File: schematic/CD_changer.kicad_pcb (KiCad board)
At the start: 2 copper layers, 27 parts, among them J1 Mini-ISO_Conn, J2 Prog, SW1 Enable, SW2 SW_Reset, U1 ESP32-WROOM-32, U3 PCM5102A

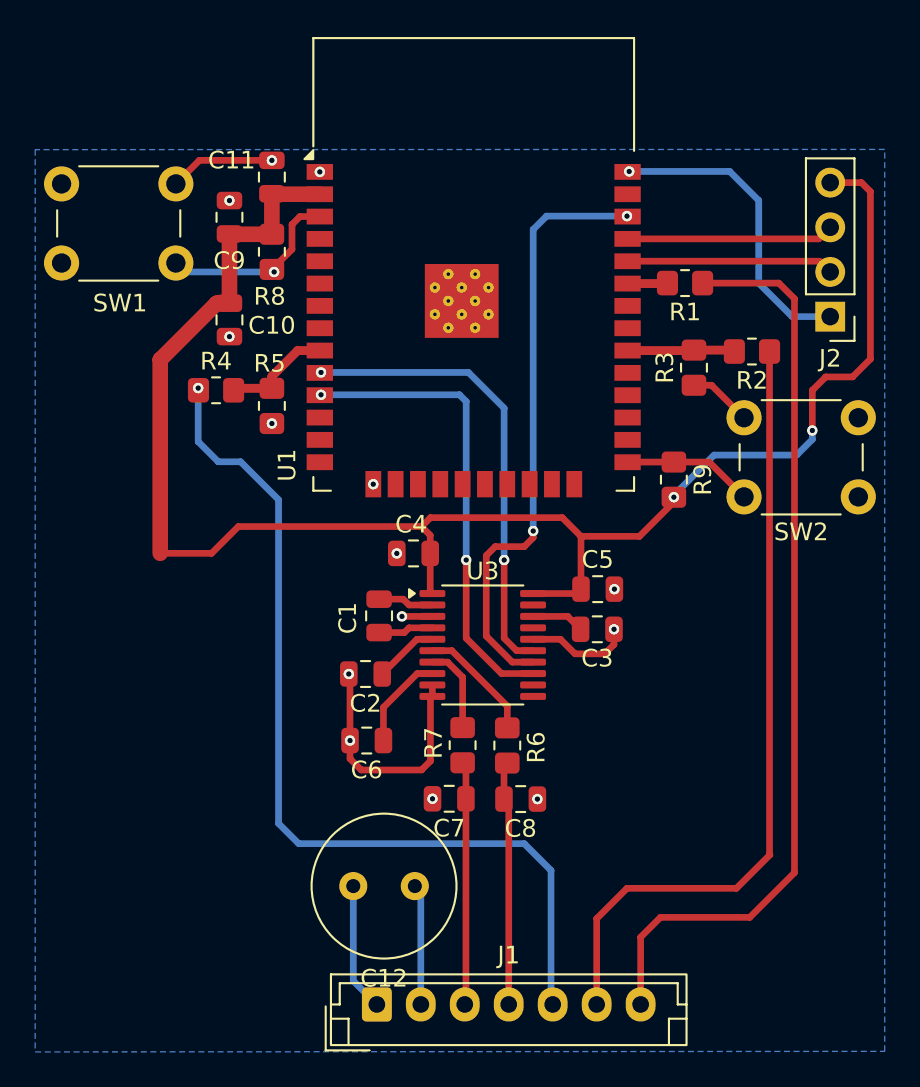
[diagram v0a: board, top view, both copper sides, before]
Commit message: Add power supply & PDF with schematic
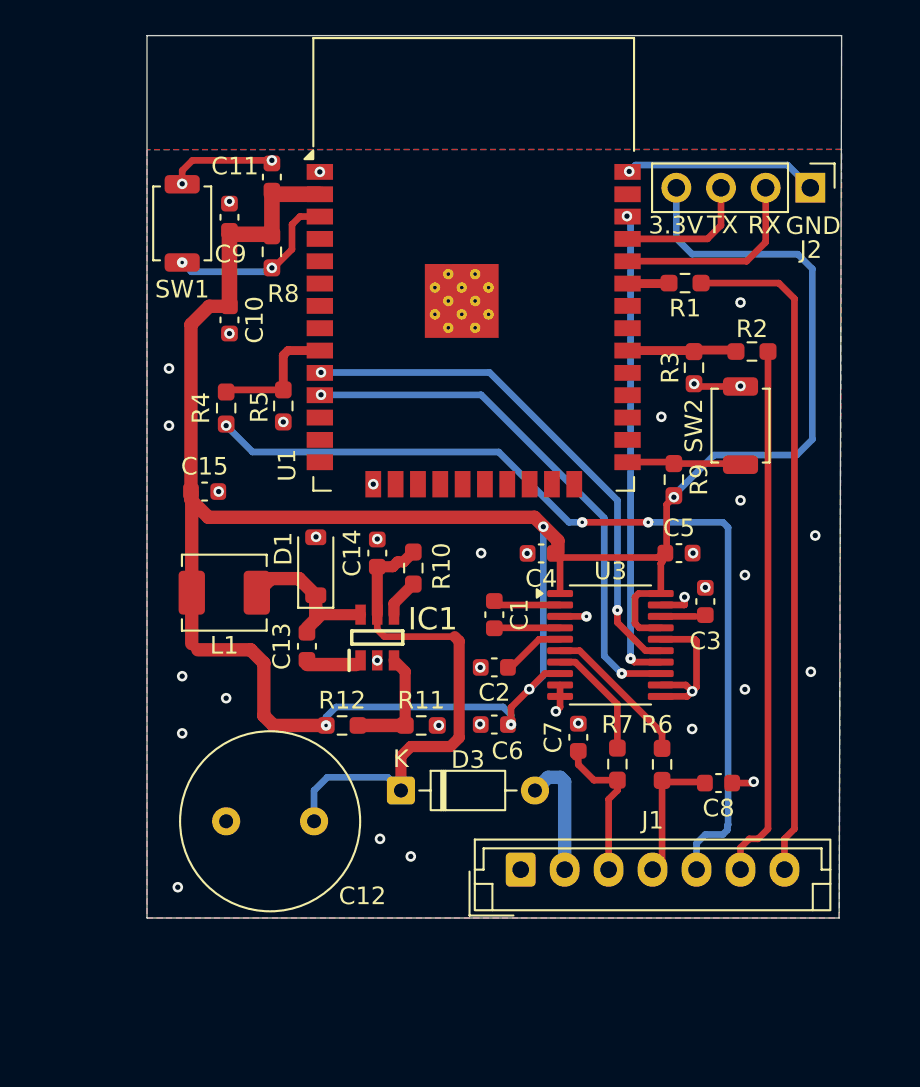
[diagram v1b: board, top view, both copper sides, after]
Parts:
- added C13: 22nF, Capacitor_SMD:C_0603_1608Metric, F.Cu at (143.3, 109.3)
- added C14: 10uF, Capacitor_SMD:C_0603_1608Metric, F.Cu at (147.3, 104.0)
- added C15: 22uF, Capacitor_SMD:C_0603_1608Metric, F.Cu at (137.5, 100.5)
- added D1: B230A, Diode_SMD:D_SOD-123, F.Cu at (143.8, 104.8)
- added D3: 1N4007, Diode_THT:D_DO-35_SOD27_P7.62mm_Horizontal, F.Cu at (148.7, 117.5)
- added IC1: MP2359DJ-LF-P, custom:SOT95P280X100-6N, F.Cu at (147.3, 108.8)
- added L1: 4.7uH, Inductor_SMD:L_Chilisin_BMRA00040420, F.Cu at (138.6, 106.2)
- added R10: 100k, Resistor_SMD:R_0603_1608Metric_Pad0.98x0.95mm_HandSolder, F.Cu at (149.4, 104.8)
- added R11: 16.2k, Resistor_SMD:R_0603_1608Metric_Pad0.98x0.95mm_HandSolder, F.Cu at (149.8, 113.8)
- added R12: 49.9k, Resistor_SMD:R_0603_1608Metric_Pad0.98x0.95mm_HandSolder, F.Cu at (145.3, 113.8)
- C1, C10, C11, C2, C3, C4, C5, C6, C7, C8, C9: footprint Capacitor_SMD:C_0805_2012Metric -> Capacitor_SMD:C_0603_1608Metric
- C12: footprint Capacitor_THT:C_Radial_D8.0mm_H7.0mm_P3.50mm -> Capacitor_THT:C_Radial_D10.0mm_H12.5mm_P5.00mm
- R1, R2, R3, R4, R5, R6, R7, R8, R9: footprint Resistor_SMD:R_0805_2012Metric_Pad1.20x1.40mm_HandSolder -> Resistor_SMD:R_0603_1608Metric_Pad0.98x0.95mm_HandSolder
- SW1, SW2: footprint Button_Switch_THT:SW_PUSH_6mm -> Button_Switch_SMD:SW_SPST_TS-1088-xR020
- moved C8 11.3 mm to (166.8, 117.1)
- moved J1 11.2 mm to (155.5, 122.0)
- moved R6 8.87 mm to (163.5, 116.0)
- moved R7 8.87 mm to (161.0, 116.0)
- moved C7 8.13 mm to (158.8, 114.5), turned to 90 degrees
- moved SW2 7.83 mm to (168.0, 96.8), turned to 90 degrees
- moved J2 7.41 mm to (172.0, 83.2), turned to -90 degrees
- moved C2 7.33 mm to (154.0, 110.5)
- moved C6 7.31 mm to (154.0, 113.8)
- moved C4 7.26 mm to (156.7, 104.0)
- moved U3 7.26 mm to (160.6, 109.2)
- moved SW1 7.22 mm to (136.2, 85.2), turned to -90 degrees
- moved C12 6.81 mm to (143.8, 119.2)
- moved C1 6.55 mm to (154.0, 107.5)
- moved C3 6.34 mm to (166.0, 106.8), turned to 90 degrees
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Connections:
- C12 pad 1: +12V -> Net-(D3-K)
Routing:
- net 3.3V: track 102.9 -> 141.9 mm, vias 2 -> 5
- net Net-(D3-K): track 0.00 -> 29.4 mm
- net GND: track 56.7 -> 35.0 mm, vias 15 -> 43
- net Net-(J1-Pin_6): track 44.9 -> 30.4 mm
- net Net-(J1-Pin_7): track 52.3 -> 38.3 mm
- net Net-(D1-K): track 0.00 -> 8.80 mm
- net DIN: track 34.1 -> 27.0 mm
- net Net-(IC1-FB): track 0.00 -> 6.46 mm
- net A_left: track 13.9 -> 7.64 mm
- net A_right: track 13.8 -> 8.91 mm
- net Net-(J2-Pin_3): track 11.8 -> 7.77 mm
- net BCK: track 26.5 -> 30.5 mm
- net WS: track 26.3 -> 29.9 mm
- net Net-(D2-K): track 0.00 -> 3.15 mm
- net Net-(IC1-EN): track 0.00 -> 2.19 mm
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- added copper zone on F.Cu, net GND
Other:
- board outline added: 39.5 x 50.2 mm
- board text added: "3.3V"
- board text added: "39.4mm"
- board text added: "50.12mm"
- board text added: "GND"
- board text added: "RX"
- board text added: "TX"
